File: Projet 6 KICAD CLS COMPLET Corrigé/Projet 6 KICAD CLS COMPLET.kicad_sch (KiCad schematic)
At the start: 16 parts, among them J1 Raspberry Pi Zero 2w, J2 Conn_01x06, J3 Screw_Terminal_01x04, J4 Screw_Terminal_01x04, J5 Battery

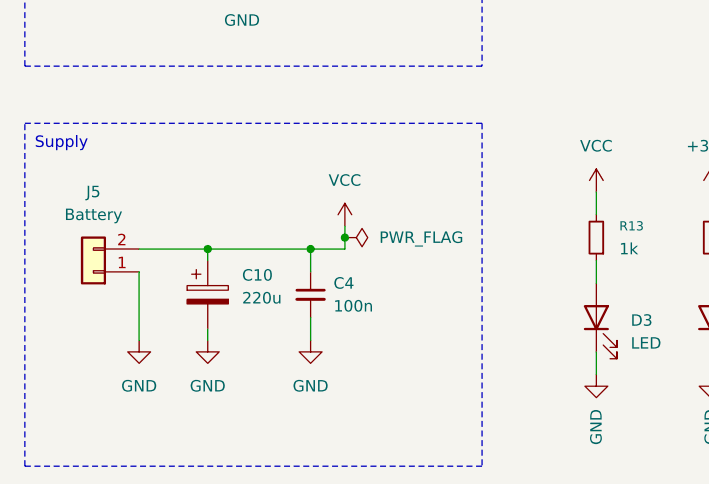
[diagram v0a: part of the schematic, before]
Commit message: Add files via upload
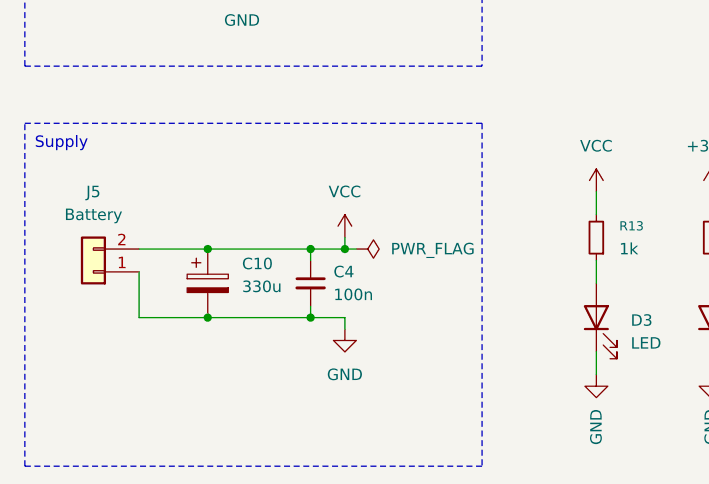
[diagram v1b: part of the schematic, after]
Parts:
- C10: value 220u -> 330u; footprint (none) -> Capacitor_SMD:CP_Elec_6.3x5.4
- C18, C4: footprint (none) -> Capacitor_SMD:C_0805_2012Metric
- D3, D4: footprint (none) -> LED_SMD:LED_0603_1608Metric
- H1, H2, H3, H4: footprint (none) -> MountingHole:MountingHole_2.7mm_M2.5_Pad
- J1: footprint (none) -> Connector_PinSocket_2.54mm:PinSocket_2x20_P2.54mm_Vertical
- J2: footprint (none) -> Connector_JST:JST_PH_B6B-PH-K_1x06_P2.00mm_Vertical
- J3, J4: footprint (none) -> Connector_JST:JST_PH_B4B-PH-K_1x04_P2.00mm_Vertical
- J5: footprint (none) -> Connector_JST:JST_EH_B2B-EH-A_1x02_P2.50mm_Vertical
- R13, R14: footprint (none) -> Resistor_SMD:R_0603_1608Metric
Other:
- moved on the sheet: C10, C4
